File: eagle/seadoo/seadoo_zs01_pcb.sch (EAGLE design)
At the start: 18 parts, among them Q1 IRFB7430PBF

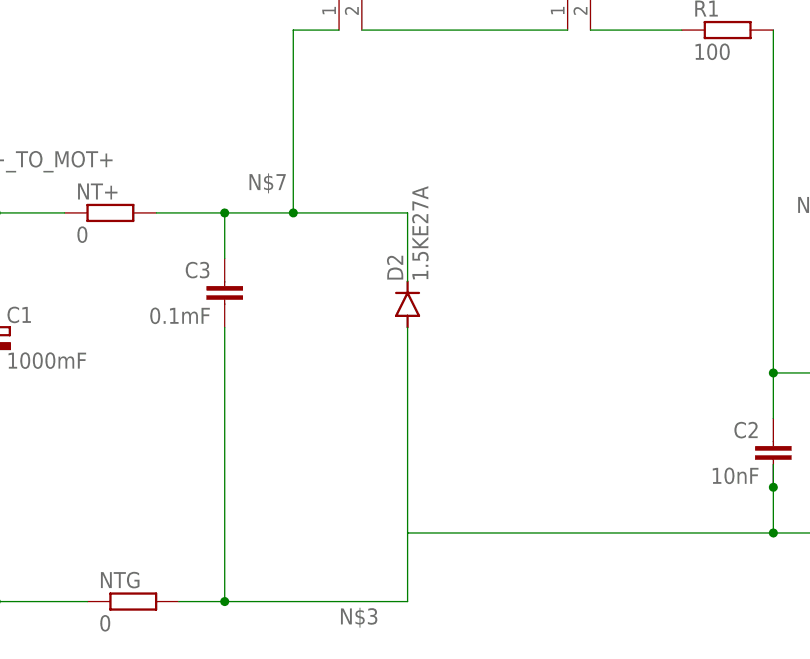
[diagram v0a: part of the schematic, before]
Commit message: As sent off for first fabrication
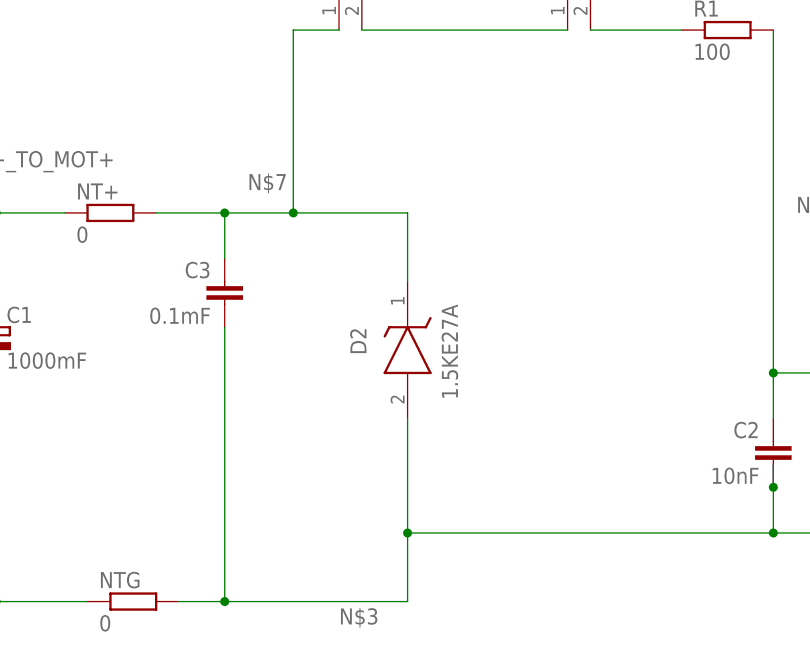
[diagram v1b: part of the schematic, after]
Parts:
- D2: device diode:DIODE-D-12.5 -> 1.5KE27A:1.5KE27A
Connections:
- net N$7: now also D2.K; no longer D2.C
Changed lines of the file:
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@@
 <part name="D1" library="diode" library_urn="urn:adsk.eagle:library:210" deviceset="DIODE-" device="TO220H" package3d_urn="urn:adsk.eagle:package:43370/1" value="VT4045BP-M3/4W"/>
 <part name="C1" library="rcl" library_urn="urn:adsk.eagle:library:334" deviceset="CPOL-EU" device="TT5D11" package3d_urn="urn:adsk.eagle:package:23309/1" value="1000mF"/>
-<part name="D2" library="diode" library_urn="urn:adsk.eagle:library:210" deviceset="DIODE-" device="D-12.5" package3d_urn="urn:adsk.eagle:package:43427/1" value="1.5KE27A"/>
 <part name="Q1" library="transistor-power" library_urn="urn:adsk.eagle:library:400" deviceset="PMOSFET_N" device="TO220BH" package3d_urn="urn:adsk.eagle:package:29490/1" value="IRFB7430PBF"/>
 <part name="S1" library="59170-1-S-00-D" deviceset="59170-1-S-00-D" device=""/>
@@
 <part name="NTG" library="rcl" library_urn="urn:adsk.eagle:library:334" deviceset="R-EU_" device="R1218" package3d_urn="urn:adsk.eagle:package:26131/2" value="0"/>
 <part name="NT+" library="rcl" library_urn="urn:adsk.eagle:library:334" deviceset="R-EU_" device="R1218" package3d_urn="urn:adsk.eagle:package:26131/2" value="0"/>
+<part name="D2" library="1.5KE27A" deviceset="1.5KE27A" device=""/>
 </parts>
 <sheets>
@@
 <attribute name="VALUE" x="8.763" y="43.6626" size="1.778" layer="96"/>
 </instance>
-<instance part="D2" gate="G$1" x="53.34" y="50.8" smashed="yes" rot="R90">
-<attribute name="NAME" x="52.8574" y="53.34" size="1.778" layer="95" rot="R90"/>
-<attribute name="VALUE" x="55.6514" y="53.34" size="1.778" layer="96" rot="R90"/>
-</instance>
 <instance part="Q1" gate="G$1" x="127" y="45.72" smashed="yes" rot="R90">
 <attribute name="NAME" x="124.46" y="50.8" size="1.778" layer="95" rot="R90"/>
@@
 <attribute name="NAME" x="16.51" y="62.4586" size="1.778" layer="95"/>
 <attribute name="VALUE" x="16.51" y="57.658" size="1.778" layer="96"/>
+</instance>
+<instance part="D2" gate="G$1" x="53.34" y="53.34" smashed="yes" rot="R270">
+<attribute name="NAME" x="46.99" y="48.26" size="1.778" layer="95" rot="R270"/>
+<attribute name="VALUE" x="57.15" y="50.8" size="1.778" layer="96" rot="R270"/>
 </instance>
 </instances>
@@
 <junction x="33.02" y="17.78"/>
 <wire x1="33.02" y1="17.78" x2="53.34" y2="17.78" width="0.1524" layer="91"/>
-<pinref part="D2" gate="G$1" pin="A"/>
-<wire x1="53.34" y1="48.26" x2="53.34" y2="25.4" width="0.1524" layer="91"/>
 <wire x1="27.94" y1="17.78" x2="33.02" y2="17.78" width="0.1524" layer="91"/>
 <pinref part="R2" gate="G$1" pin="1"/>
@@
 <wire x1="119.38" y1="30.48" x2="119.38" y2="25.4" width="0.1524" layer="91"/>
 <pinref part="NTG" gate="G$1" pin="2"/>
+<pinref part="D2" gate="G$1" pin="A"/>
+<wire x1="53.34" y1="38.1" x2="53.34" y2="25.4" width="0.1524" layer="91"/>
+<junction x="53.34" y="25.4"/>
 </segment>
 </net>
@@
 <pinref part="S1" gate="G$1" pin="1"/>
 <wire x1="40.64" y1="81.28" x2="45.72" y2="81.28" width="0.1524" layer="91"/>
-<pinref part="D2" gate="G$1" pin="C"/>
-<wire x1="53.34" y1="53.34" x2="53.34" y2="60.96" width="0.1524" layer="91"/>
 <wire x1="40.64" y1="60.96" x2="53.34" y2="60.96" width="0.1524" layer="91"/>
 <label x="35.56" y="63.5" size="1.778" layer="95"/>
@@
 <junction x="33.02" y="60.96"/>
 <pinref part="NT+" gate="G$1" pin="2"/>
-</segment>
-</net>
+<pinref part="D2" gate="G$1" pin="K"/>
+<wire x1="53.34" y1="60.96" x2="53.34" y2="53.34" width="0.1524" layer="91"/>
+</segment>
+</net>
